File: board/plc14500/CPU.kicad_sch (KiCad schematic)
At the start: 78 parts, among them U10 MC14500, U11 74HC14, U3 74HC14, U7 74HC590A, U8 LH5168, U9 NE555

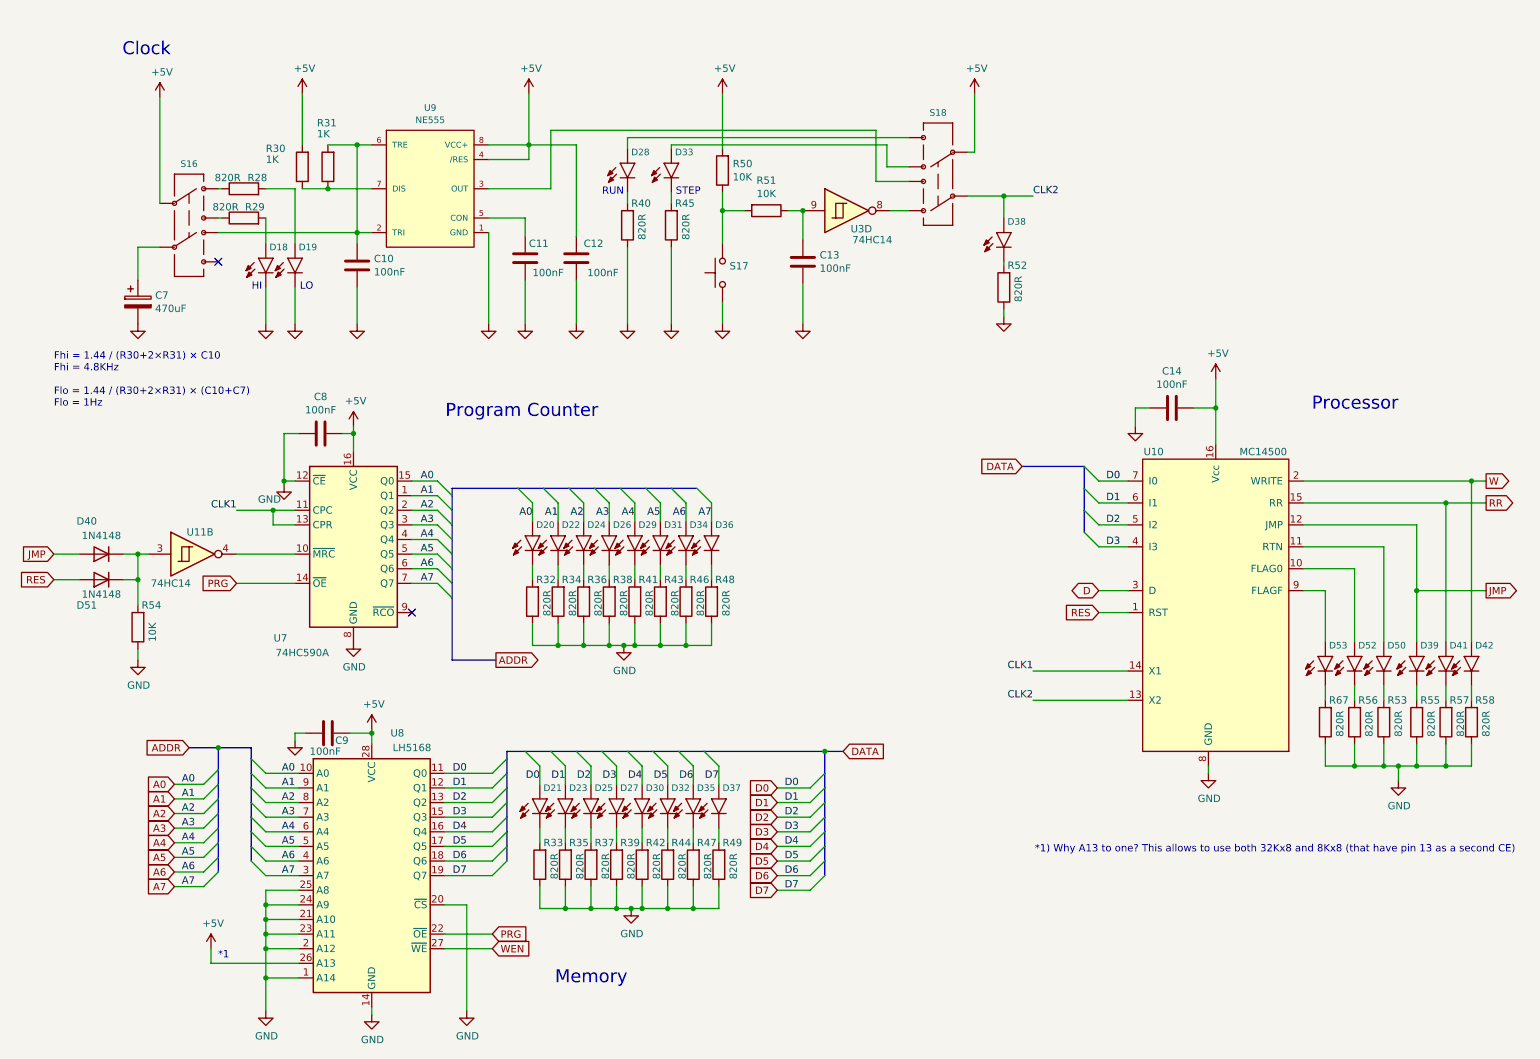
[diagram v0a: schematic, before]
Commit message: REV.D Schema updates
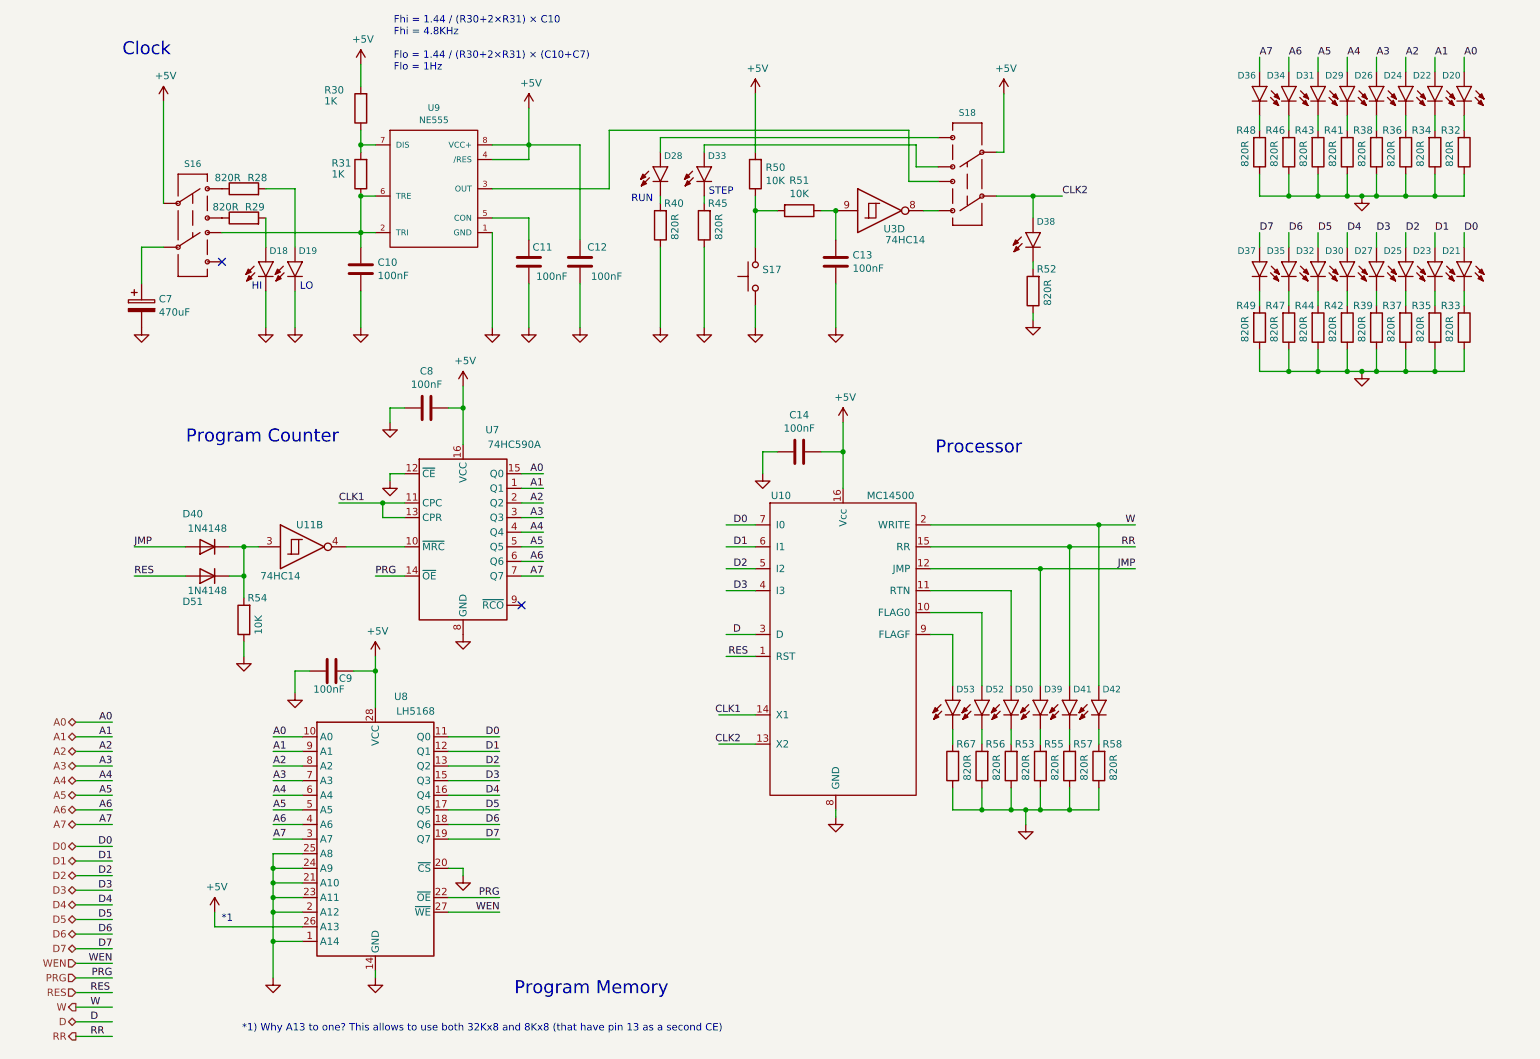
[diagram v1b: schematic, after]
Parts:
- S16, S18: symbol plc14500-rescue:SWITCH-DPDT-PTH-GPI-152-3013-SparkFun-Switches -> plc14500:SWITCH-DPDT
- U11, U3: symbol 74xx:74HC14 -> plc14500:74HC14
- U7: symbol 74xx:74HC590A -> plc14500:74HC590A
- U8: symbol Memory_RAM:KM62256CLP -> plc14500:KM62256CLP
- U9: symbol plc14500-rescue:555D-SparkFun-IC-Special-Function -> plc14500:555
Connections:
- net at R30.1, U9.7 (DIS): now also R31.2; no longer R31.1
- net at C10.1, U9.2 (TRI), U9.6 (TRE): now also R31.1, S16.7; no longer R31.2, S16.5
- net at U9.3 (OUT): now also S18.1; no longer S18.3
- net at U3.8: now also S18.3; no longer S18.1
- net at S18.5: now also D28.A; no longer D33.A
- net at S18.7: now also D33.A; no longer D28.A
- net at S16.1: now also R29.1; no longer R28.1
- net at S16.3: now also R28.1; no longer R29.1
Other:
- note added: "Program Memory"
- note removed: "Memory"
- moved on the sheet: C10, C11, C12, C13, C14, C7, C8, C9, D18, D19, D20, D21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
